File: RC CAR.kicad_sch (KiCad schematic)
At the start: 11 parts, among them J1 RW, J2 LW, J4 US, J5 RGB, J6 J2, J7 J2, U1 L293D, U2 ESP32-DEVKIT-V1, U3 L7805

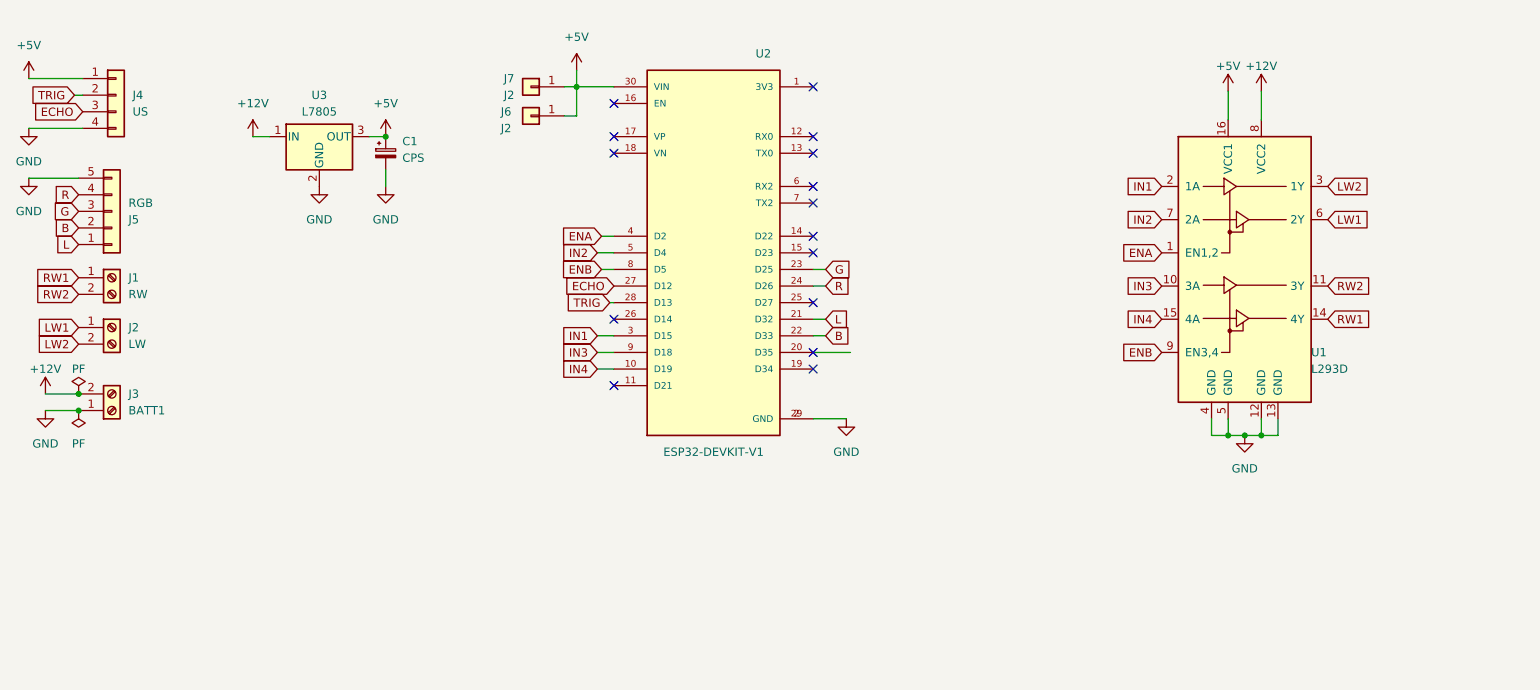
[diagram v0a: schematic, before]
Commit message: Raspberry Pico Dev-Board Copy
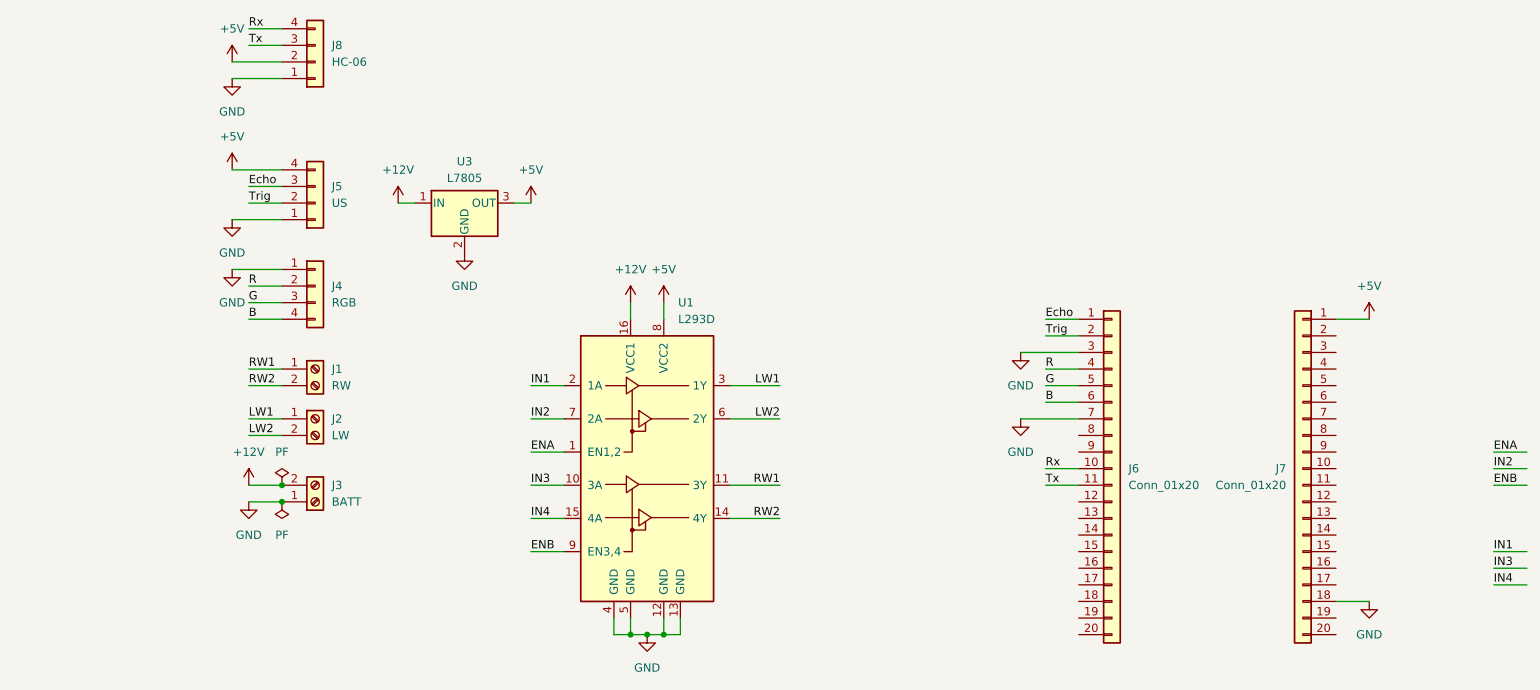
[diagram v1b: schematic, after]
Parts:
- removed C1: CPS, Capacitor_THT:CP_Radial_D5.0mm_P2.50mm, symbol Device:C_Polarized_Small
- removed J5: RGB, Connector_PinSocket_2.54mm:PinSocket_1x05_P2.54mm_Horizontal, symbol Connector_Generic:Conn_01x05
- removed J6, J7: J2, Connector_PinHeader_2.54mm:PinHeader_1x01_P2.54mm_Vertical, symbol Connector_Generic:Conn_01x01
- removed U2: ESP32-DEVKIT-V1, MODULE_ESP32_DEVKIT_V1:MODULE_ESP32_DEVKIT_V1, symbol ESP32-DEVKIT-V1:ESP32-DEVKIT-V1
- added J4: RGB, Connector_PinHeader_2.54mm:PinHeader_1x04_P2.54mm_Vertical, symbol Connector_Generic:Conn_01x04
- added J6, J7: Conn_01x20, Connector_PinHeader_2.54mm:PinHeader_1x20_P2.54mm_Vertical, symbol Connector_Generic:Conn_01x20
- added J8: HC-06, Connector_PinSocket_2.54mm:PinSocket_1x04_P2.54mm_Horizontal, symbol Connector_Generic:Conn_01x04
- J1, J2: footprint TerminalBlock:TerminalBlock_Altech_AK300-2_P5.00mm -> TerminalBlock_4Ucon:TerminalBlock_4Ucon_1x02_P3.50mm_Horizontal
- J3: renamed from BATT1; value J3 -> BATT; footprint TerminalBlock:TerminalBlock_Altech_AK300-2_P5.00mm -> TerminalBlock_4Ucon:TerminalBlock_4Ucon_1x02_P3.50mm_Horizontal
- J5: renamed from J4; footprint Connector_PinHeader_2.54mm:PinHeader_1x04_P2.54mm_Horizontal -> Connector_PinHeader_2.54mm:PinHeader_1x04_P2.54mm_Vertical
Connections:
- net +12V: now also U1.16 (VCC1); no longer U1.8 (VCC2)
- net +5V: now also J5.4 (Pin_4), U1.8 (VCC2), J7.1 (Pin_1), J8.2 (Pin_2); no longer J5.1 (Pin_1), U1.16 (VCC1)
- net B: now also J4.4 (Pin_4), J6.6 (Pin_6)
- net G: now also J4.3 (Pin_3), J6.5 (Pin_5)
- net GND: now also J5.1 (Pin_1), J4.1 (Pin_1), J6.3 (Pin_3), J6.7 (Pin_7), J7.18 (Pin_18), J8.1 (Pin_1); no longer J5.4 (Pin_4)
- net LW1: now also U1.3 (1Y); no longer U1.6 (2Y)
- net LW2: now also U1.6 (2Y); no longer U1.3 (1Y)
- net R: now also J4.2 (Pin_2), J6.4 (Pin_4)
- net RW1: now also U1.11 (3Y); no longer U1.14 (4Y)
- net RW2: now also U1.14 (4Y); no longer U1.11 (3Y)
- net ECHO renamed Echo
- net Echo: now also J6.1 (Pin_1)
- net TRIG renamed Trig
- net Trig: now also J6.2 (Pin_2)
- new net Rx: J6.10 (Pin_10), J8.4 (Pin_4)
- new net Tx: J6.11 (Pin_11), J8.3 (Pin_3)
- no-connect marks 15 -> 0
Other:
- moved on the sheet: J1, J2, J3, J5, U1, U3
